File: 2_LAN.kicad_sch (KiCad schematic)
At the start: 56 parts, among them U1 LAN9514, U5 M93C86-WMN6TP, X1 25MHz

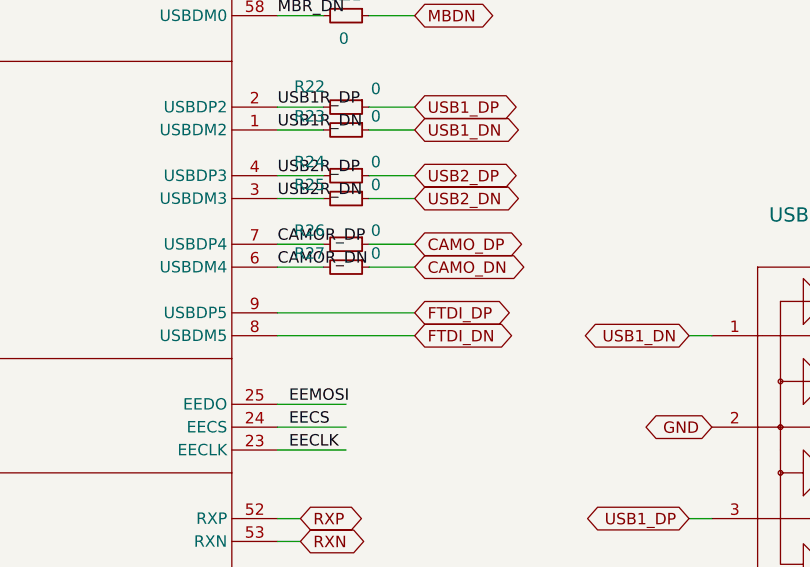
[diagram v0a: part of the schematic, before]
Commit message: WIP: move passives around for U1
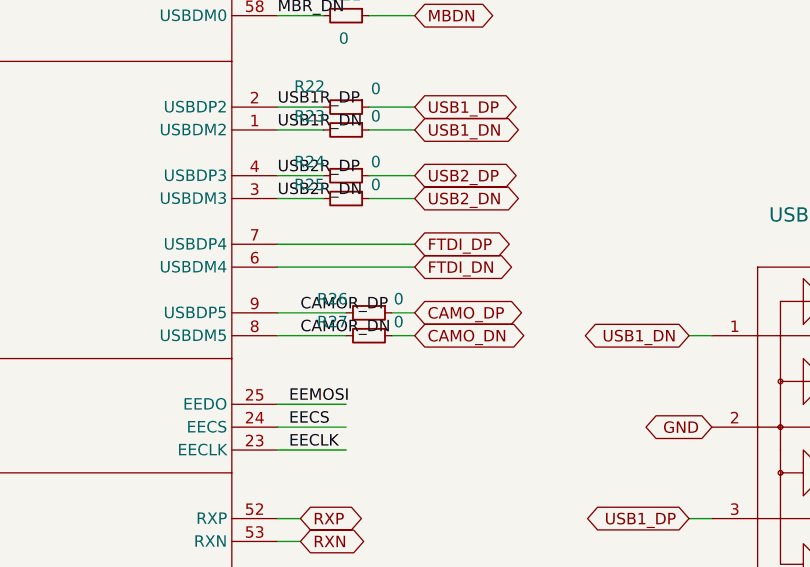
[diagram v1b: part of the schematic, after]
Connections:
- net CAMOR_DN: now also U1.8 (USBDM5); no longer U1.6 (USBDM4)
- net CAMOR_DP: now also U1.9 (USBDP5); no longer U1.7 (USBDP4)
- net FTDI_DN: now also U1.6 (USBDM4); no longer U1.8 (USBDM5)
- net FTDI_DP: now also U1.7 (USBDP4); no longer U1.9 (USBDP5)
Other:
- moved on the sheet: R26, R27
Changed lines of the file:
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@@
 	(wire
 		(pts
-			(xy 147.32 93.98) (xy 162.56 93.98)
+			(xy 184.15 27.94) (xy 191.77 27.94)
 		)
 		(stroke
@@
 	(wire
 		(pts
-			(xy 184.15 27.94) (xy 191.77 27.94)
+			(xy 157.48 58.42) (xy 162.56 58.42)
 		)
 		(stroke
@@
 	(wire
 		(pts
-			(xy 157.48 58.42) (xy 162.56 58.42)
+			(xy 66.04 11.43) (xy 66.04 17.78)
 		)
 		(stroke
@@
 	(wire
 		(pts
-			(xy 66.04 11.43) (xy 66.04 17.78)
+			(xy 147.32 83.82) (xy 162.56 83.82)
 		)
 		(stroke
@@
 	(wire
 		(pts
-			(xy 147.32 83.82) (xy 152.4 83.82)
-		)
-		(stroke
-			(width 0)
-			(type default)
-		)
-	)
-	(wire
-		(pts
 			(xy 179.07 176.53) (xy 179.07 180.34)
 		)
@@
 	(wire
 		(pts
+			(xy 147.32 91.44) (xy 154.94 91.44)
+		)
+		(stroke
+			(width 0)
+			(type default)
+		)
+	)
+	(wire
+		(pts
 			(xy 147.32 20.32) (xy 147.32 22.86)
 		)
@@
 	(wire
 		(pts
-			(xy 153.67 27.94) (xy 161.29 27.94)
+			(xy 147.32 93.98) (xy 154.94 93.98)
 		)
 		(stroke
@@
 	(wire
 		(pts
-			(xy 191.77 26.67) (xy 191.77 27.94)
+			(xy 153.67 27.94) (xy 161.29 27.94)
 		)
 		(stroke
@@
 	(wire
 		(pts
-			(xy 63.5 175.26) (xy 63.5 172.72)
+			(xy 191.77 26.67) (xy 191.77 27.94)
 		)
 		(stroke
@@
 	(wire
 		(pts
-			(xy 147.32 91.44) (xy 162.56 91.44)
+			(xy 63.5 175.26) (xy 63.5 172.72)
 		)
 		(stroke
@@
 	(wire
 		(pts
-			(xy 157.48 86.36) (xy 162.56 86.36)
+			(xy 160.02 93.98) (xy 162.56 93.98)
 		)
 		(stroke
@@
 	(wire
 		(pts
-			(xy 147.32 86.36) (xy 152.4 86.36)
-		)
-		(stroke
-			(width 0)
-			(type default)
-		)
-	)
-	(wire
-		(pts
 			(xy 30.48 96.52) (xy 38.1 96.52)
 		)
@@
 	(wire
 		(pts
-			(xy 157.48 83.82) (xy 162.56 83.82)
+			(xy 160.02 91.44) (xy 162.56 91.44)
 		)
 		(stroke
@@
 	(wire
 		(pts
+			(xy 147.32 86.36) (xy 162.56 86.36)
+		)
+		(stroke
+			(width 0)
+			(type default)
+		)
+	)
+	(wire
+		(pts
 			(xy 256.54 167.64) (xy 260.35 167.64)
 		)
@@
 	)
 	(label "CAMOR_DP"
-		(at 147.32 83.82 0)
+		(at 149.86 91.44 0)
 		(fields_autoplaced yes)
 		(effects
@@
 	)
 	(label "CAMOR_DN"
-		(at 147.32 86.36 0)
+		(at 149.86 93.98 0)
 		(fields_autoplaced yes)
 		(effects
@@
 	(global_label "CAMO_DN"
 		(shape bidirectional)
-		(at 162.56 86.36 0)
+		(at 162.56 93.98 0)
 		(effects
 			(font
@@
 		)
 		(property "Intersheetrefs" "${INTERSHEET_REFS}"
-			(at 162.56 86.36 0)
+			(at 162.56 93.98 0)
 			(effects
 				(font
@@
 	(global_label "FTDI_DP"
 		(shape bidirectional)
-		(at 162.56 91.44 0)
+		(at 162.56 83.82 0)
 		(effects
 			(font
@@
 		)
 		(property "Intersheetrefs" "${INTERSHEET_REFS}"
-			(at 162.56 91.44 0)
+			(at 162.56 83.82 0)
 			(effects
 				(font
@@
 	(global_label "CAMO_DP"
 		(shape bidirectional)
-		(at 162.56 83.82 0)
+		(at 162.56 91.44 0)
 		(effects
 			(font
@@
 		)
 		(property "Intersheetrefs" "${INTERSHEET_REFS}"
-			(at 162.56 83.82 0)
+			(at 162.56 91.44 0)
 			(effects
 				(font
@@
 	(global_label "FTDI_DN"
 		(shape bidirectional)
-		(at 162.56 93.98 0)
+		(at 162.56 86.36 0)
 		(effects
 			(font
@@
 		)
 		(property "Intersheetrefs" "${INTERSHEET_REFS}"
-			(at 162.56 93.98 0)
+			(at 162.56 86.36 0)
 			(effects
 				(font
@@
 	(symbol
 		(lib_id "Device:R_Small")
-		(at 154.94 86.36 270)
+		(at 157.48 93.98 270)
 		(unit 1)
 		(exclude_from_sim no)
@@
 		(dnp no)
 		(property "Reference" "R27"
-			(at 150.876 84.836 90)
+			(at 153.416 92.456 90)
 			(effects
 				(font
@@
 		)
 		(property "Value" "0"
-			(at 158.242 84.836 90)
+			(at 160.782 92.456 90)
 			(effects
 				(font
@@
 		)
 		(property "Footprint" "Resistor_SMD:R_0603_1608Metric"
-			(at 154.94 86.36 0)
+			(at 157.48 93.98 0)
 			(effects
 				(font
@@
 		)
 		(property "Datasheet" "~"
-			(at 154.94 86.36 0)
+			(at 157.48 93.98 0)
 			(effects
 				(font
@@
 		)
 		(property "Description" "Resistor, small symbol"
-			(at 154.94 86.36 0)
+			(at 157.48 93.98 0)
 			(effects
 				(font
@@
 		)
 		(property "LCSC" "C21189"
-			(at 150.876 84.836 0)
+			(at 153.416 92.456 0)
 			(effects
 				(font
@@
 	(symbol
 		(lib_id "Device:R_Small")
-		(at 154.94 83.82 270)
+		(at 157.48 91.44 270)
 		(unit 1)
 		(exclude_from_sim no)
@@
 		(dnp no)
 		(property "Reference" "R26"
-			(at 150.876 82.296 90)
+			(at 153.416 89.916 90)
 			(effects
 				(font
@@
 		)
 		(property "Value" "0"
-			(at 158.242 82.296 90)
+			(at 160.782 89.916 90)
 			(effects
 				(font
@@
 		)
 		(property "Footprint" "Resistor_SMD:R_0603_1608Metric"
-			(at 154.94 83.82 0)
+			(at 157.48 91.44 0)
 			(effects
 				(font
@@
 		)
 		(property "Datasheet" "~"
-			(at 154.94 83.82 0)
+			(at 157.48 91.44 0)
 			(effects
 				(font
@@
 		)
 		(property "Description" "Resistor, small symbol"
-			(at 154.94 83.82 0)
+			(at 157.48 91.44 0)
 			(effects
 				(font
@@
 		)
 		(property "LCSC" "C21189"
-			(at 150.876 82.296 0)
+			(at 153.416 89.916 0)
 			(effects
 				(font
